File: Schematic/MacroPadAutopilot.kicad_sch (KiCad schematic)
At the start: 23 parts, among them J1 OLED_Display, SW1 CherryMX, SW10 RotaryEncoder, SW2 CherryMX, SW3 CherryMX, SW4 CherryMX, SW5 CherryMX, SW6 CherryMX, SW7 SW_SPDT, SW8 RotaryEncoder, SW9 RotaryEncoder

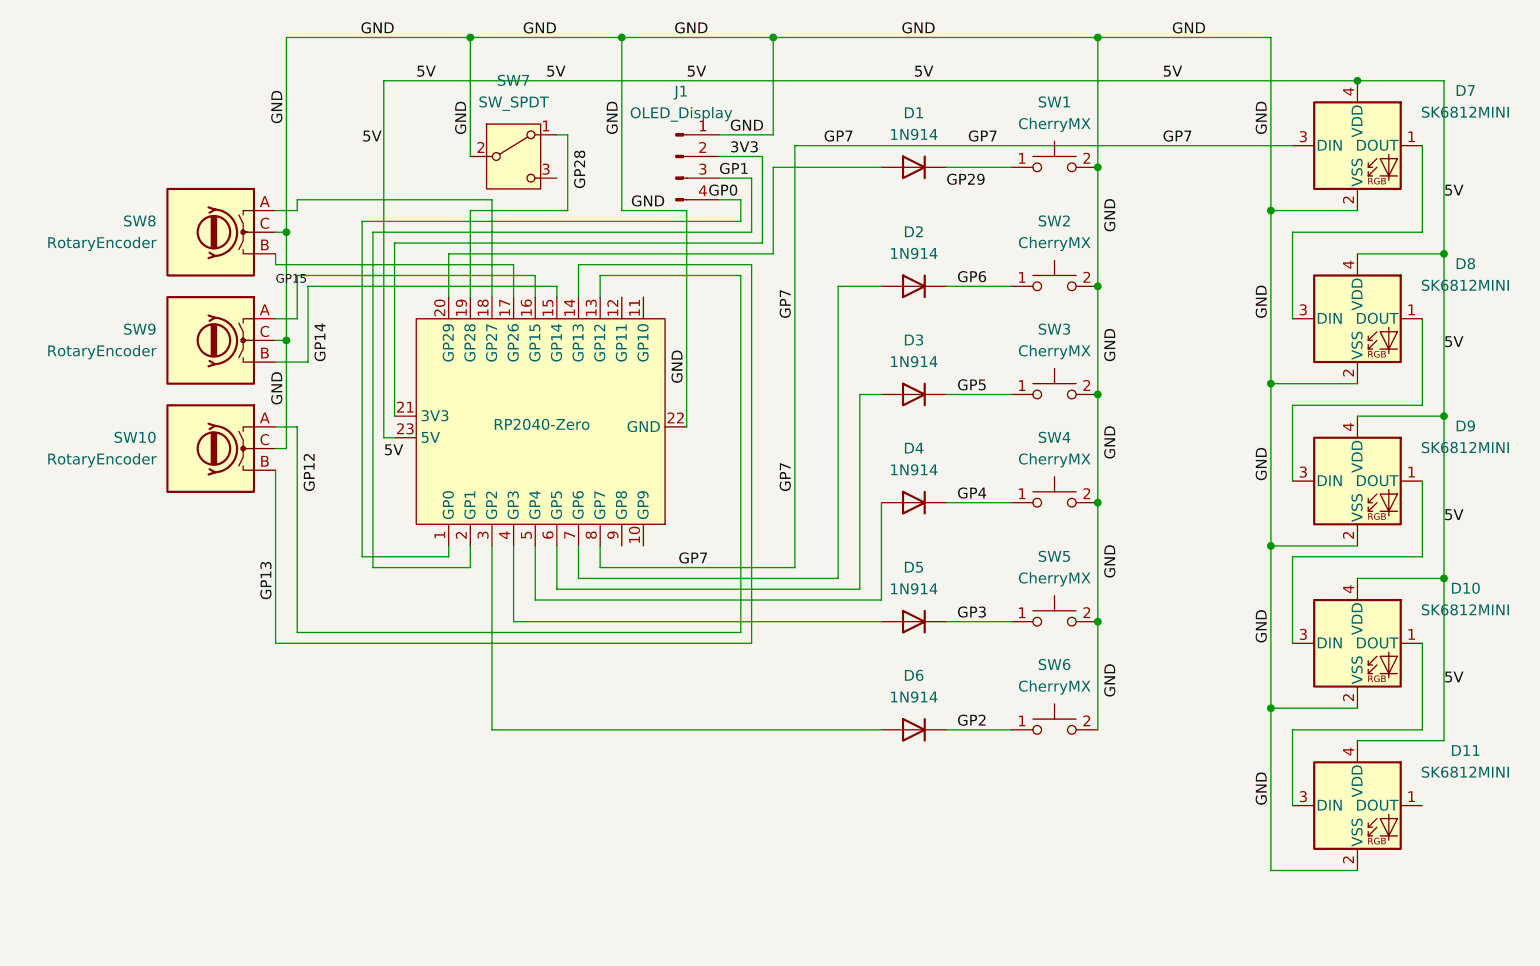
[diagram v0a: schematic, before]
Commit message: Add files via upload
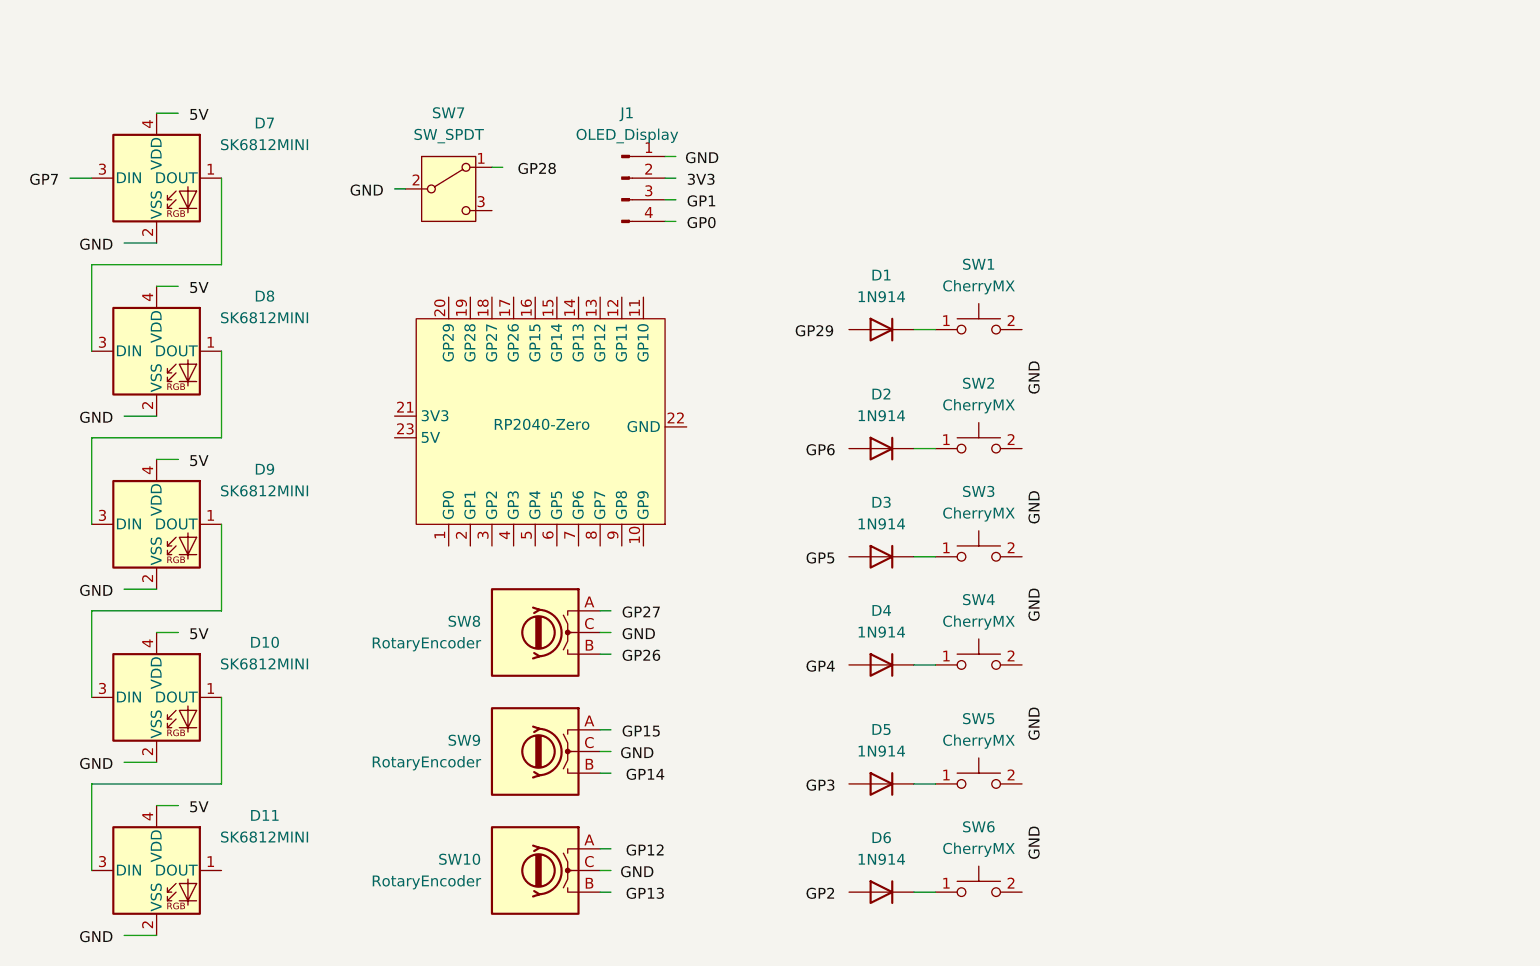
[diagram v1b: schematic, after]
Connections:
- net 3V3: no longer J1.2 (Pin_2), RZ1.21 (3V3)
- net 5V: no longer D10.4 (VDD), D11.4 (VDD), D7.4 (VDD), D8.4 (VDD), D9.4 (VDD), RZ1.23 (5V)
- net GND: no longer D10.2 (VSS), D11.2 (VSS), D7.2 (VSS), D8.2 (VSS), D9.2 (VSS), J1.1 (Pin_1), RZ1.22 (GND), SW1.2, SW10.C, SW2.2, SW3.2, SW4.2, SW5.2, SW6.2, SW7.2 (B), SW8.C, SW9.C
- net GP1: no longer J1.3 (Pin_3), RZ1.2 (GP1)
- net GP13: no longer RZ1.14 (GP13), SW10.B
- net GP2: no longer D6.1 (K), SW6.1
- net GP3: no longer D5.1 (K), SW5.1
- net GP4: no longer D4.1 (K), SW4.1
- net GP5: no longer D3.1 (K), SW3.1
- net GP6: no longer D2.1 (K), SW2.1
- net GP7: no longer D7.3 (DIN), RZ1.8 (GP7)
- net at SW10.A: no longer RZ1.13 (GP12)
- net at SW7.1 (A): no longer RZ1.19 (GP28)
- net at D1.2 (A): no longer RZ1.20 (GP29)
- net at RZ1.1 (GP0): no longer J1.4 (Pin_4)
- net at RZ1.15 (GP14): no longer SW9.B
- net at RZ1.16 (GP15): no longer SW9.A
- net at RZ1.17 (GP26): no longer SW8.B
- net at RZ1.18 (GP27): no longer SW8.A
- net at RZ1.3 (GP2): no longer D6.2 (A)
- net at RZ1.4 (GP3): no longer D5.2 (A)
- net at RZ1.5 (GP4): no longer D4.2 (A)
- net at RZ1.6 (GP5): no longer D3.2 (A)
- net at RZ1.7 (GP6): no longer D2.2 (A)
- new net: D2.1 (K), SW2.1
- new net: D4.1 (K), SW4.1
- new net: D6.1 (K), SW6.1
- new net: D3.1 (K), SW3.1
- new net: D5.1 (K), SW5.1
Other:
- moved on the sheet: D1, D10, D11, D2, D3, D4, D5, D6, D7, D8, D9, J1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
